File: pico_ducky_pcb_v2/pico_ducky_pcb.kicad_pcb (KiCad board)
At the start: 4 copper layers, 14 x 30 mm, 32 parts, among them J1 USB_A, J3 Conn_ARM_JTAG_SWD_10, SW1 R-667799, SW2 R-667799, U1 AP2127K-3.3, U2 W25Q32JVZP, U3 RP2040, Y1 Crystal_GND24

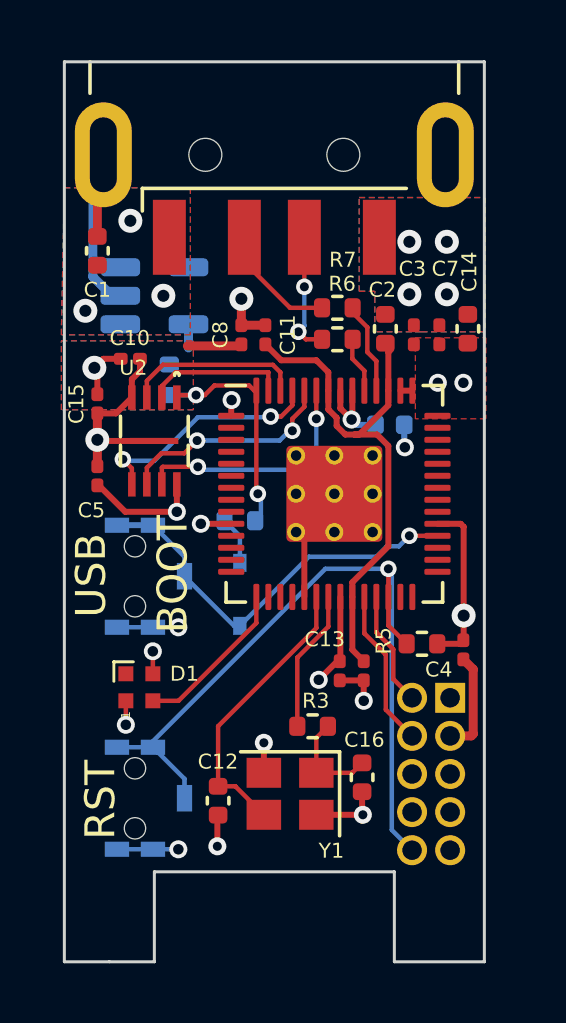
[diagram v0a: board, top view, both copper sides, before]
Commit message: route out most of the pcb
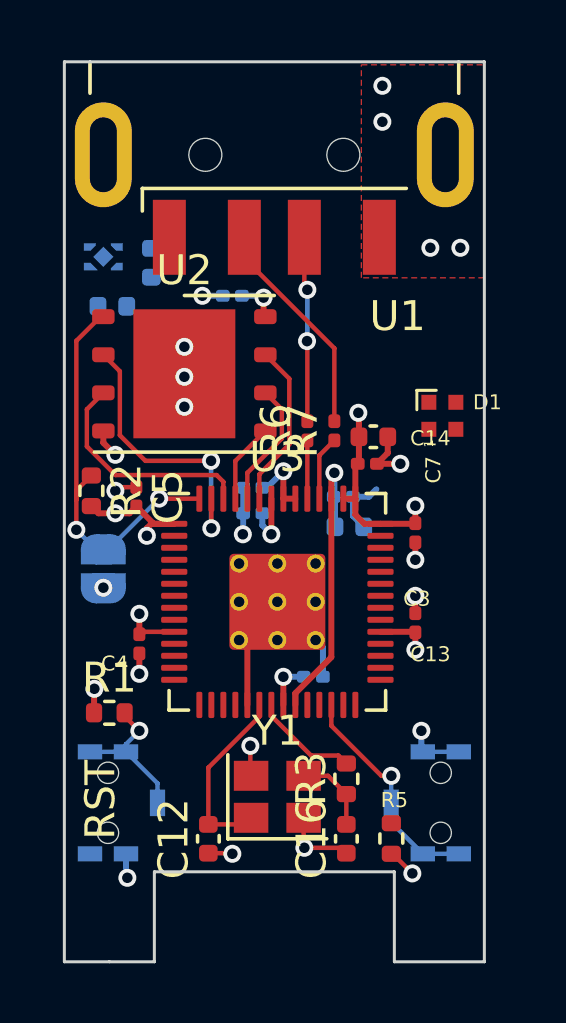
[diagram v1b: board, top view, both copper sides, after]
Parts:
- removed D2: NSR0320, Diode_SMD:D_SOD-323
- removed J3: Conn_ARM_JTAG_SWD_10, Connector_PinHeader_1.27mm:PinHeader_2x05_P1.27mm_Vertical
- removed R4: 1k, Resistor_SMD:R_0402_1005Metric
- added JP1: SolderJumper_2_Open, Jumper:SolderJumper-2_P1.3mm_Open_RoundedPad1.0x1.5mm, B.Cu at (81.3, 56.9)
- added R1: 10k, Resistor_SMD:R_0402_1005Metric, F.Cu at (81.5, 61.7)
- C1, C10, C11, C15, C2, C8, C9: moved to B.Cu
- R2: moved to F.Cu
- R6, R7: footprint Resistor_SMD:R_0402_1005Metric -> Resistor_SMD:R_0201_0603Metric
- U1: value AP2127K-3.3 -> MIC5504-3.3YM5; footprint Package_TO_SOT_SMD:SOT-23-5 -> Package_DFN_QFN:UDFN-4-1EP_1x1mm_P0.65mm_EP0.48x0.48mm
- U2: footprint 8-UFDFN:W25Q80DVUXIE TR -> Package_SON:WSON-8-1EP_6x5mm_P1.27mm_EP3.4x4.3mm
- moved D1 13.6 mm to (92.6, 51.8)
- moved C8 11.6 mm to (88.3, 60.5), turned to 180 degrees
- moved C4 10.8 mm to (82.5, 59.4)
- moved SW2 10.7 mm to (92.8, 64.7), turned to -90 degrees
- moved C6 9.61 mm to (82.9, 46.7), turned to 90 degrees
- moved SW1 7.60 mm to (81.2, 64.7)
- moved C2 6.71 mm to (89.5, 55.5), turned to 180 degrees
- moved C3 6.60 mm to (91.7, 55.7), turned to 90 degrees
- moved R5 6.57 mm to (90.9, 65.9), turned to 90 degrees
- moved C11 5.96 mm to (86.3, 55.0), turned to 0 degrees
- moved C15 5.89 mm to (86.3, 54.2), turned to 0 degrees
- moved C9 5.84 mm to (89.3, 54.5), turned to 180 degrees
- moved C7 4.92 mm to (90.1, 53.4), turned to 180 degrees
- moved C14 4.78 mm to (90.3, 52.5), turned to 180 degrees
- moved R2 4.52 mm to (80.9, 54.3), turned to -90 degrees
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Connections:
- SW1 pad B1: /USB_BOOT -> /SAFE_BOOT
- SW1 pad B2: /USB_BOOT -> /SAFE_BOOT
- SW1 pad B3: /USB_BOOT -> /SAFE_BOOT
- Y1 pad 1: Net-(C16-Pad2) -> /X_IN
- Y1 pad 3: /X_IN -> Net-(C16-Pad2)
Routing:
- net /RESET: track 26.2 -> 7.62 mm
- net /USB_BOOT: track 13.7 -> 0.00 mm, vias 1 -> 0
- net GND: track 32.6 -> 20.3 mm, vias 14 -> 21
- net /QSPI_CS: track 7.95 -> 13.6 mm
- net +1V1: track 17.7 -> 12.2 mm, vias 0 -> 2
- net /RGB_DI: track 5.39 -> 0.00 mm
- net /SWCLK: track 5.29 -> 0.00 mm
- net /QSPI_SD0: track 7.83 -> 2.67 mm, vias 2 -> 0
- net /SAFE_BOOT: track 0.00 -> 5.02 mm, vias 0 -> 1
- net /QSPI_SD1: track 4.73 -> 9.55 mm, vias 0 -> 2
- net /USB_-: track 3.22 -> 7.37 mm
- net /SWD: track 3.86 -> 0.00 mm
- net /X_IN: track 9.59 -> 6.20 mm
- net /QSPI_SCLK: track 7.42 -> 4.23 mm, vias 2 -> 0
- net /QSPI_SD3: track 8.12 -> 5.54 mm, vias 2 -> 0
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- removed copper zone on B.Cu, net +3V3
- removed copper zone on F.Cu, net +3V3
- removed copper zone on B.Cu, net +5V
- removed copper zone on F.Cu, net +5V
- removed copper zone on B.Cu, net GND
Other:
- board text removed: "BOOT"
- board text removed: "RP Duck V1"
- board text removed: "USB"
